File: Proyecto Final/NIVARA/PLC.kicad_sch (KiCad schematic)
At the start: 11 parts, among them J1 Screw_Terminal_2_P5.00mm, J13 Screw_Terminal_4_P5.00mm, J2 Screw_Terminal_2_P5.00mm, J3 Screw_Terminal_2_P5.00mm, J4 Screw_Terminal_2_P5.00mm, J5 Screw_Terminal_6_P5.00mm, J6 Screw_Terminal_4_P5.00mm, J7 Screw_Terminal_3_P5.00mm, J8 Screw_Terminal_3_P5.00mm, J9 Screw_Terminal_2_P5.00mm

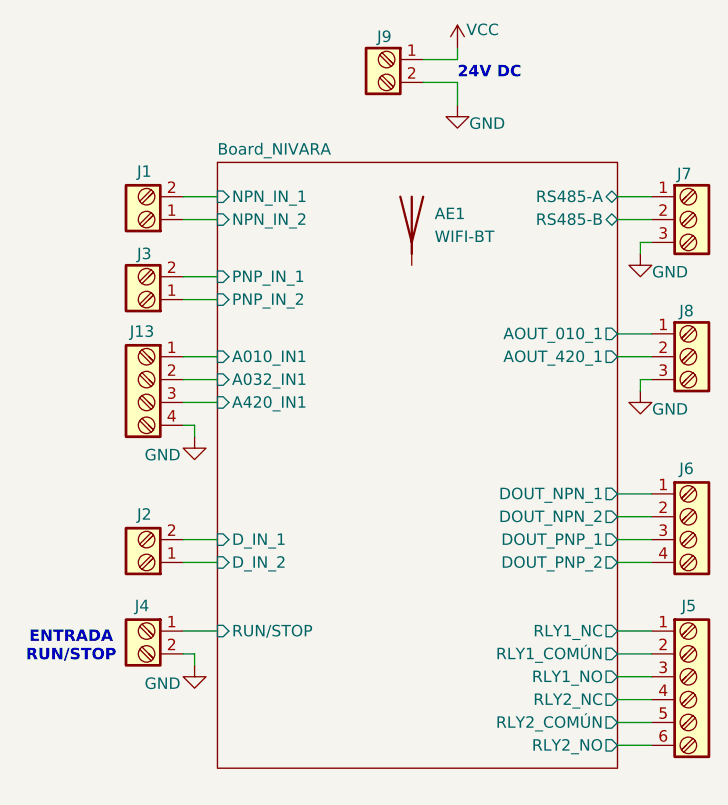
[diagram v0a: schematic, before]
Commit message: Actualización
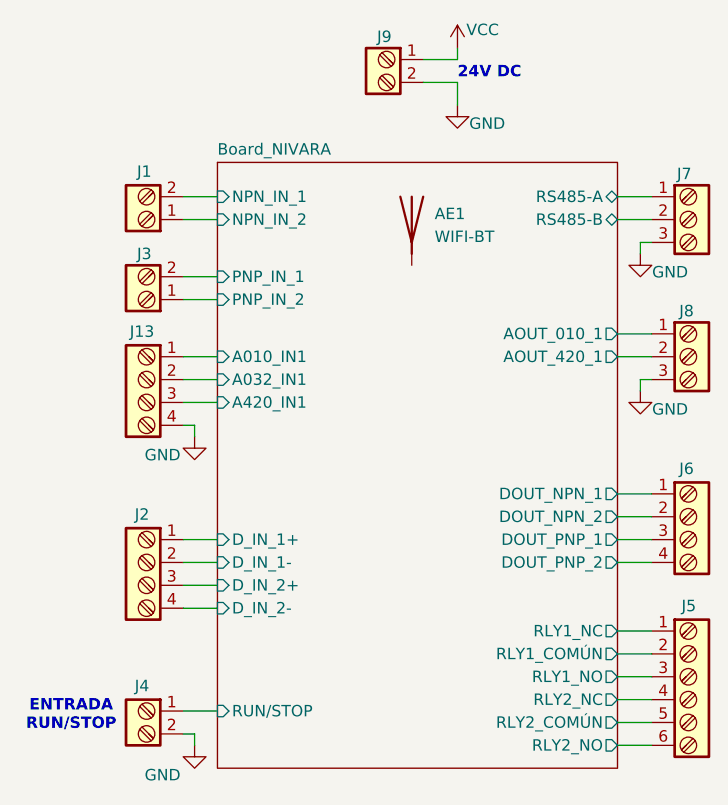
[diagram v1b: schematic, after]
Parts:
- removed J2: Screw_Terminal_2_P5.00mm, TerminalBlock_Phoenix:TerminalBlock_Phoenix_PT-1,5-2-5.0-H_1x02_P5.00mm_Horizontal, symbol PCM_SL_Screw_Terminal:Screw_Terminal_2_P5.00mm
- added J2: Screw_Terminal_4_P5.00mm, TerminalBlock_Phoenix:TerminalBlock_Phoenix_PT-1,5-4-5.0-H_1x04_P5.00mm_Horizontal, symbol PCM_SL_Screw_Terminal:Screw_Terminal_4_P5.00mm
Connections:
- new net Board_NIVARA/D_IN_1+: J2.1
- new net Board_NIVARA/D_IN_1-: J2.2
- new net Board_NIVARA/D_IN_2+: J2.3
- new net Board_NIVARA/D_IN_2-: J2.4
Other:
- sheet Board_NIVARA ports: added D_IN_1+, D_IN_1-, D_IN_2+, D_IN_2-; removed D_IN_1, D_IN_2
- moved on the sheet: J4
